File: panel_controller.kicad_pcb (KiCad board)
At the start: 2 copper layers, 75 x 60 mm, 9 parts, among them J1 SBH11-PBPC-D08-ST-BK, J2 215297-6, J3 Screw_Terminal_01x03, J4 Screw_Terminal_01x02, U1 ESP32-DEVKIT-V1

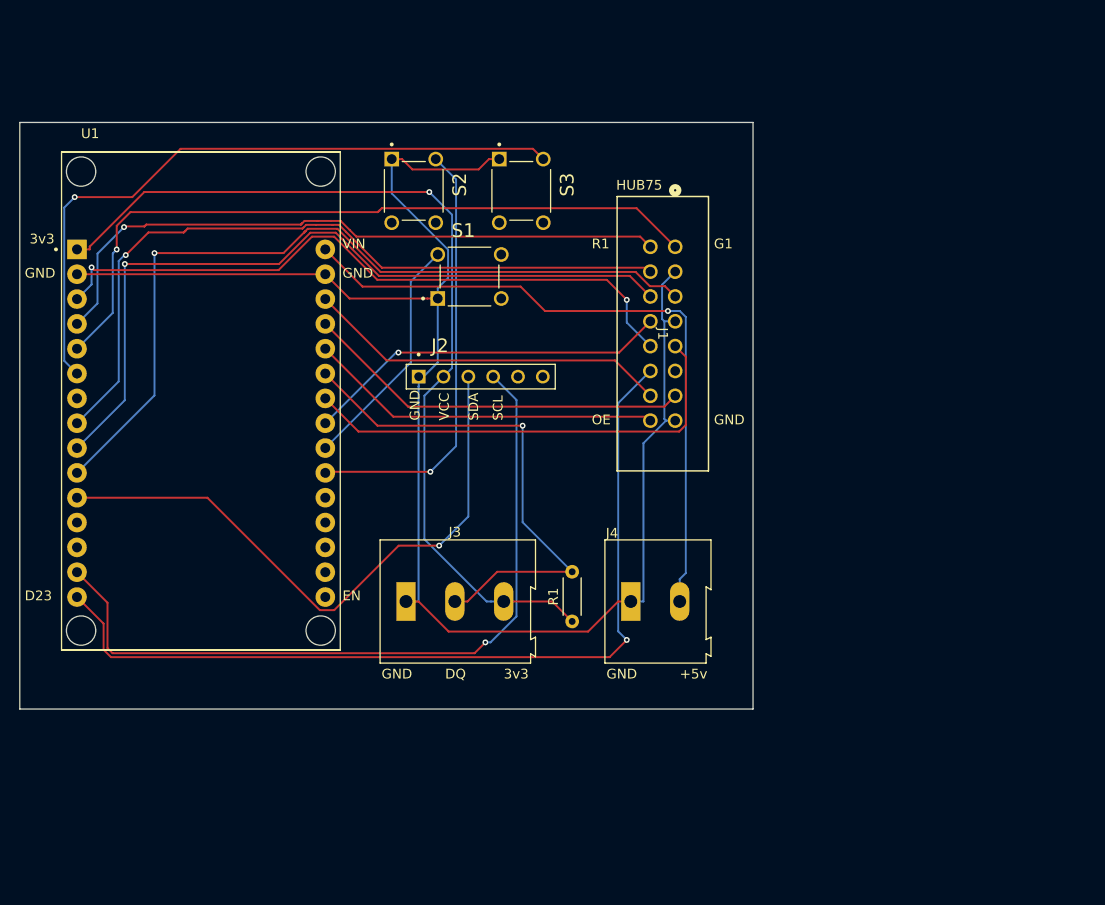
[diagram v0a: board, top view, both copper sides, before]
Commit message: pcb clock v1.1
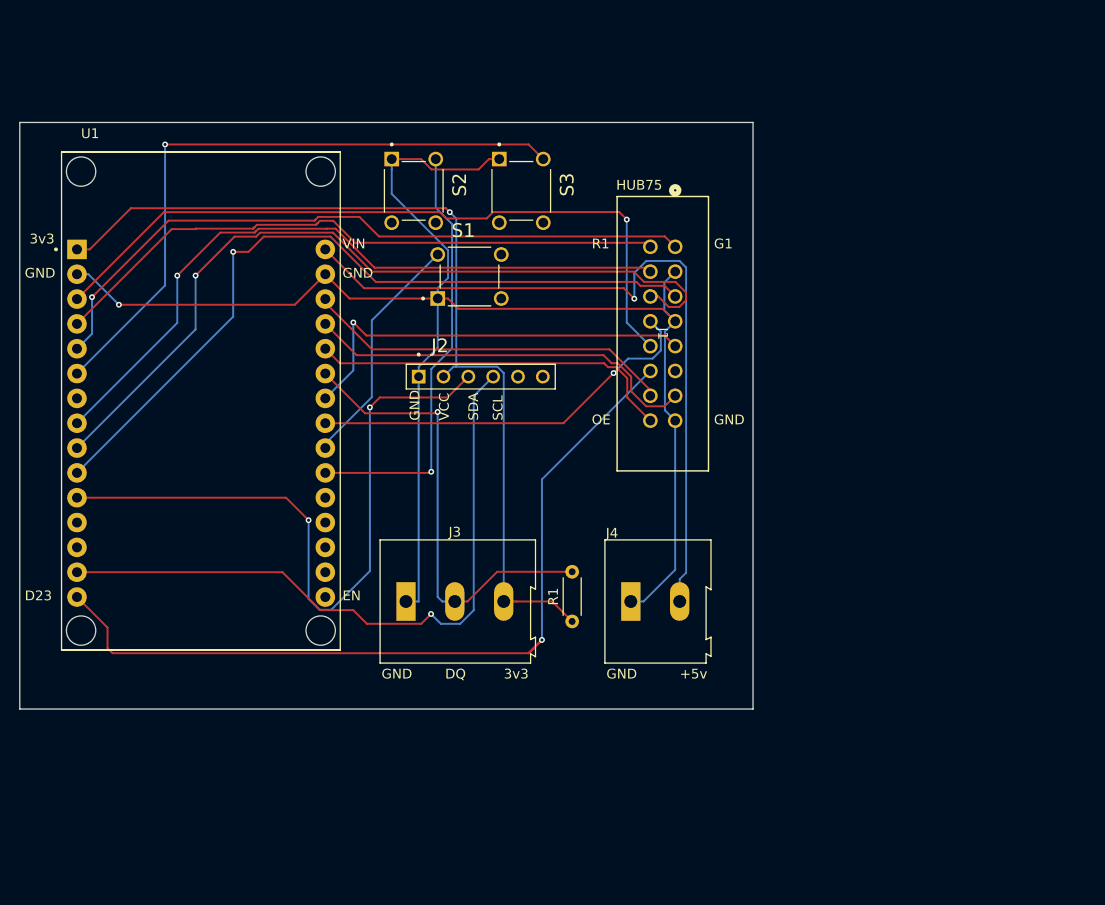
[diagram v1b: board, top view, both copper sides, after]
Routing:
- net Net-(U1-D22): track 78.2 -> 68.9 mm
- net Net-(J4-Pin_2): track 69.1 -> 76.9 mm
- net Net-(U1-D21): track 63.1 -> 69.2 mm, vias 1 -> 2
- net Net-(U1-D15): track 68.8 -> 74.7 mm, vias 2 -> 1
- net Net-(U1-D19): track 83.1 -> 77.6 mm
- net Net-(U1-D5): track 77.2 -> 71.8 mm
- net Net-(J3-Pin_2): track 52.7 -> 47.4 mm
- net Net-(U1-D26): track 47.1 -> 42.9 mm, vias 0 -> 1
- net Net-(U1-D18): track 78.6 -> 82.4 mm
- net Net-(U1-D4): track 74.1 -> 70.4 mm
- net Net-(U1-D25): track 37.6 -> 40.8 mm
- net Net-(U1-RX2): track 69.4 -> 66.5 mm
- net Net-(U1-D2): track 67.5 -> 64.7 mm, vias 1 -> 0
- net Net-(U1-D23): track 90.3 -> 91.5 mm
- net Net-(J3-Pin_1): track 164.8 -> 166.0 mm, vias 0 -> 1
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
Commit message: pcb clock v1.2
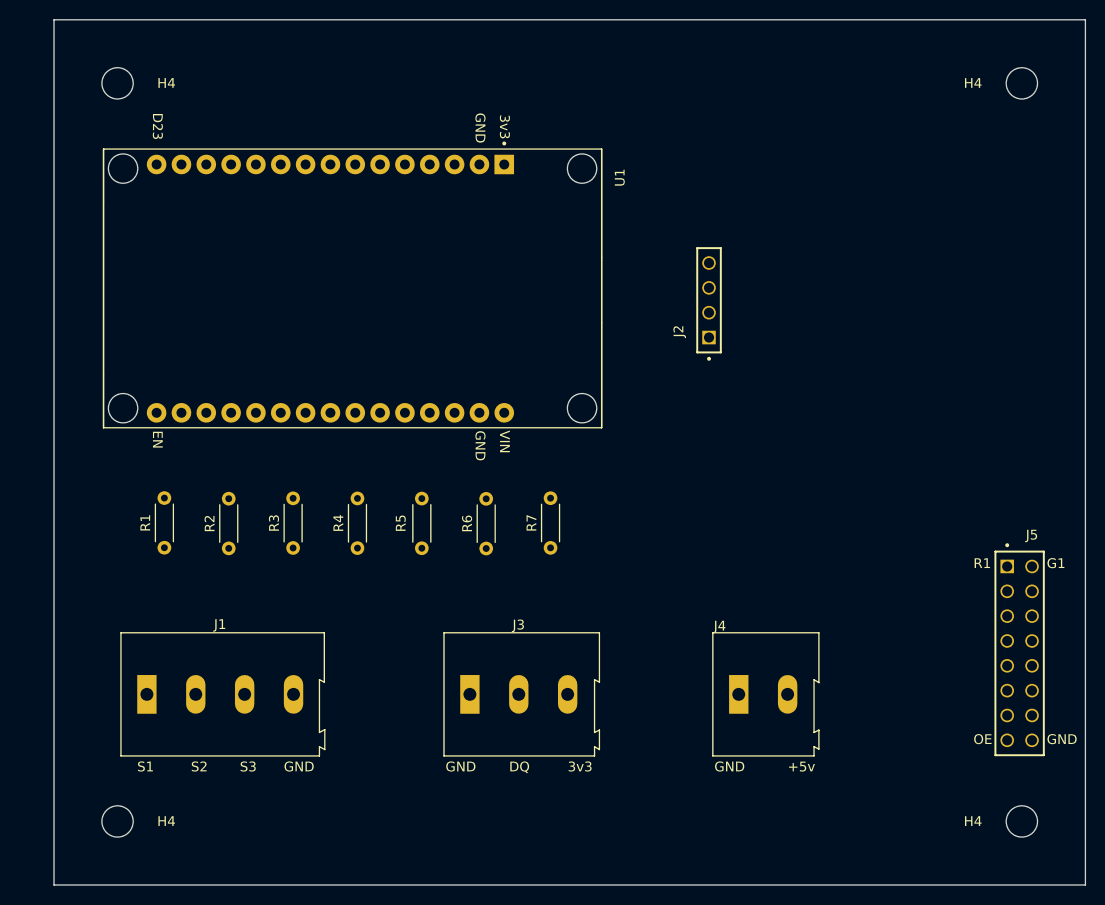
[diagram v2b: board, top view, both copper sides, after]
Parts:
- removed S1, S2, S3: TL1105YF160Q, TL1105YF160Q:SW_TL1105YF160Q
- added H4: MountingHole_3.2mm_M3, MountingHole:MountingHole_3.2mm_M3, F.Cu at (126.0, 64.0)
- added H4: MountingHole_3.2mm_M3, MountingHole:MountingHole_3.2mm_M3, F.Cu at (218.5, 139.5)
- added H4: MountingHole_3.2mm_M3, MountingHole:MountingHole_3.2mm_M3, F.Cu at (218.5, 64.0)
- added H4: MountingHole_3.2mm_M3, MountingHole:MountingHole_3.2mm_M3, F.Cu at (126.0, 139.5)
- added J5: SSW-108-02-G-D, SSW-108-02-G-D:SAMTEC_SSW-108-02-G-D, F.Cu at (227.0, 123.4)
- added R2: 1k, Resistor_THT:R_Axial_DIN0204_L3.6mm_D1.6mm_P5.08mm_Horizontal, F.Cu at (137.4, 111.6)
- added R3: 1k, Resistor_THT:R_Axial_DIN0204_L3.6mm_D1.6mm_P5.08mm_Horizontal, F.Cu at (144.0, 111.5)
- added R4: 1k, Resistor_THT:R_Axial_DIN0204_L3.6mm_D1.6mm_P5.08mm_Horizontal, F.Cu at (150.5, 111.5)
- added R5: 220, Resistor_THT:R_Axial_DIN0204_L3.6mm_D1.6mm_P5.08mm_Horizontal, F.Cu at (157.1, 111.6)
- added R6: 220, Resistor_THT:R_Axial_DIN0204_L3.6mm_D1.6mm_P5.08mm_Horizontal, F.Cu at (163.7, 111.6)
- added R7: 220, Resistor_THT:R_Axial_DIN0204_L3.6mm_D1.6mm_P5.08mm_Horizontal, F.Cu at (170.3, 111.5)
- J1: value SBH11-PBPC-D08-ST-BK -> Screw_Terminal_01x04; footprint footprints:CONN16_SBH11-PBPC-D08-ST-BK_SUL -> TerminalBlock:TerminalBlock_Altech_AK300-4_P5.00mm
- J2: value 215297-6 -> SSW-104-01-F-S; footprint 215297_6:TE_215297-6 -> SSW-104-01-F-S:SAMTEC_SSW-104-01-F-S-RTC
- moved J1 60.0 mm to (129.0, 126.5)
- moved R1 42.4 mm to (130.8, 111.5)
- moved U1 19.3 mm to (150.0, 85.0), turned to -90 degrees
- moved J2 16.3 mm to (178.0, 87.2), turned to 90 degrees
- moved J4 14.6 mm to (189.5, 126.5)
- moved J3 11.5 mm to (162.0, 126.5)
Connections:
- net Net-(J4-Pin_2) renamed +5V
- J1 pad 1: Net-(U1-D4) -> Net-(J1-Pin_1)
- J1 pad 2: Net-(U1-D2) -> Net-(J1-Pin_2)
- J1 pad 3: Net-(J3-Pin_1) -> Net-(J1-Pin_3)
- J1 pad 4: Net-(U1-D5) -> GND
- J3 pad 1: Net-(J3-Pin_1) -> GND
- J3 pad 3: Net-(J3-Pin_3) -> +3V3
- J4 pad 1: Net-(J3-Pin_1) -> GND
- R1 pad 1: Net-(J3-Pin_3) -> Net-(J3-Pin_2)
- R1 pad 2: Net-(J3-Pin_2) -> +3V3
- U1 pad 1: Net-(J3-Pin_3) -> +3V3
- U1 pad 2: Net-(J3-Pin_1) -> GND
- U1 pad 29: Net-(J3-Pin_1) -> GND
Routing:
- net Net-(J3-Pin_1): track 166.0 -> 0.00 mm, vias 1 -> 0
- net Net-(J3-Pin_3): track 94.2 -> 0.00 mm, vias 1 -> 0
- net Net-(U1-D23): track 91.5 -> 0.00 mm, vias 1 -> 0
- net Net-(U1-D18): track 82.4 -> 0.00 mm, vias 1 -> 0
- net Net-(U1-D19): track 77.6 -> 0.00 mm, vias 1 -> 0
- net +5V: track 76.9 -> 0.00 mm, vias 1 -> 0
- net Net-(U1-D15): track 74.7 -> 0.00 mm, vias 1 -> 0
- net Net-(U1-D5): track 71.8 -> 0.00 mm, vias 1 -> 0
- net Net-(U1-D4): track 70.4 -> 0.00 mm, vias 1 -> 0
- net Net-(U1-D21): track 69.2 -> 0.00 mm, vias 2 -> 0
- net Net-(U1-D22): track 68.9 -> 0.00 mm, vias 1 -> 0
- net Net-(U1-RX2): track 66.5 -> 0.00 mm, vias 1 -> 0
- net Net-(U1-D2): track 64.7 -> 0.00 mm
- net Net-(J3-Pin_2): track 47.4 -> 0.00 mm, vias 1 -> 0
- net Net-(U1-D32): track 44.4 -> 0.00 mm, vias 1 -> 0
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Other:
- board size 75 x 60 mm -> 105.5 x 88.5 mm
- board text added: "S1"
- board text added: "S2"
- board text added: "S3"
- board text removed: "HUB75"
- board text removed: "SCL"
- board text removed: "SDA"
- board text removed: "VCC"
